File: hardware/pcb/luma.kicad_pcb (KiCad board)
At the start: 2 copper layers, 40 x 58 mm, 81 parts, among them J1 Conn_01x03, J2 Conn_01x03_Pin, Q1 SS8050, Q2 SS8050, SW1 SW_Push, SW2 SW_Push, U1 ESP32-WROOM-32E(8MB), U15 FAN48610BUC50X, U2 USBLC6-2SC6, U6 CP2102N-Axx-xQFN28

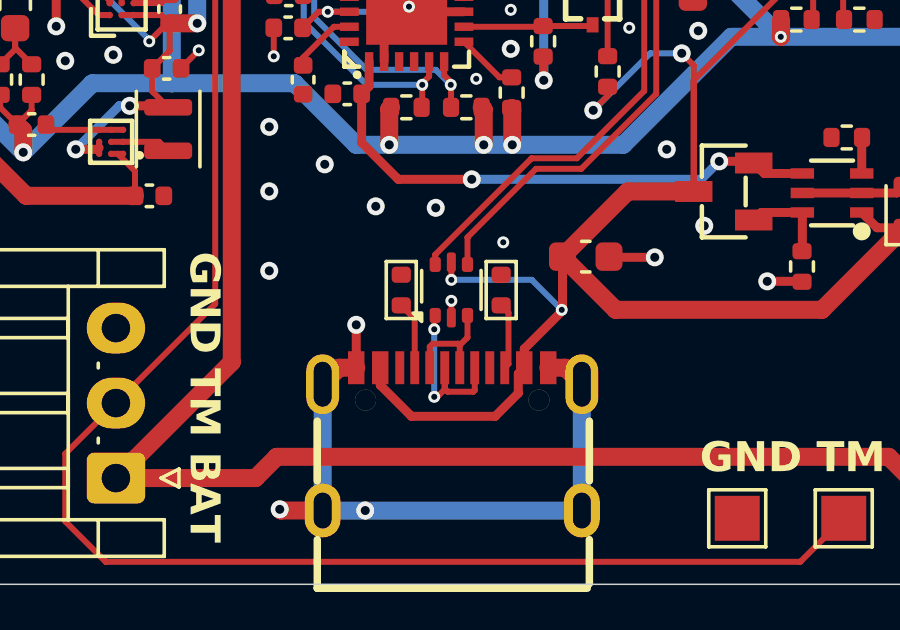
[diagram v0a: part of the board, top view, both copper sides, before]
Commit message: added tolerances an finished build
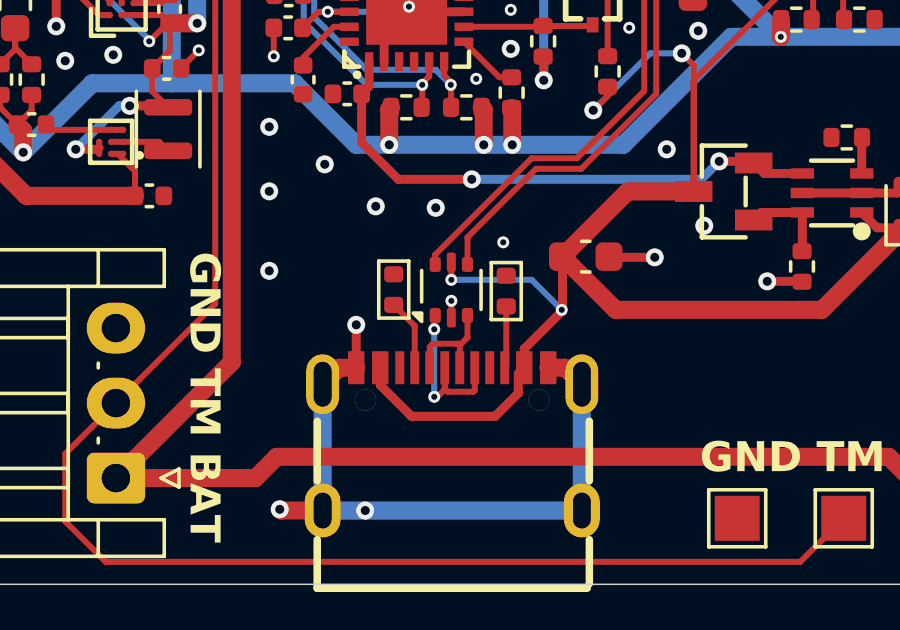
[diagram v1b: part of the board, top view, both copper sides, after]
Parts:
- moved R2 0.25 mm to (201.2, 121.5)
- moved R1 0.17 mm to (204.9, 121.5)
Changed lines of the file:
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@@
 	(footprint "PCM_Resistor_SMD_AKL:R_0402_1005Metric"
 		(layer "F.Cu")
-		(at 204.73 121.49 90)
+		(at 204.9 121.525 90)
 		(descr "Resistor SMD 0402 (1005 Metric), square (rectangular) end terminal, IPC_7351 nominal, (Body size source: IPC-SM-782 page 72, https://www.pcb-3d.com/wordpress/wp-content/uploads/ipc-sm-782a_amendment_1_and_2.pdf), Alternate KiCad Library")
 		(tags "resistor")
@@
 	(footprint "PCM_Resistor_SMD_AKL:R_0402_1005Metric"
 		(layer "F.Cu")
-		(at 201.4 121.49 90)
+		(at 201.15 121.475 90)
 		(descr "Resistor SMD 0402 (1005 Metric), square (rectangular) end terminal, IPC_7351 nominal, (Body size source: IPC-SM-782 page 72, https://www.pcb-3d.com/wordpress/wp-content/uploads/ipc-sm-782a_amendment_1_and_2.pdf), Alternate KiCad Library")
 		(tags "resistor")
@@
 	)
 	(segment
-		(start 204.85 124.08)
-		(end 204.974 123.956)
+		(start 204.9 124.03)
+		(end 204.9 122.035)
 		(width 0.2)
 		(layer "F.Cu")
@@
 	)
 	(segment
-		(start 204.974 123.956)
-		(end 204.974 122.244)
-		(width 0.2)
-		(layer "F.Cu")
-		(net 35)
-	)
-	(segment
-		(start 204.974 122.244)
-		(end 204.73 122)
+		(start 204.85 124.08)
+		(end 204.9 124.03)
 		(width 0.2)
 		(layer "F.Cu")
@@
 	)
 	(segment
-		(start 201.85 122.45)
-		(end 201.4 122)
+		(start 201.85 122.685)
+		(end 201.15 121.985)
 		(width 0.2)
 		(layer "F.Cu")
@@
 	(segment
 		(start 201.85 124.08)
-		(end 201.85 122.45)
+		(end 201.85 122.685)
 		(width 0.2)
 		(layer "F.Cu")
